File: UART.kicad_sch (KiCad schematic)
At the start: 22 parts, among them J19 430450212, J9 430450612, T1 DA2304-ALD, U5 MAX485, U6 LP2985A-50DBVR, U9 ISO3086TDW

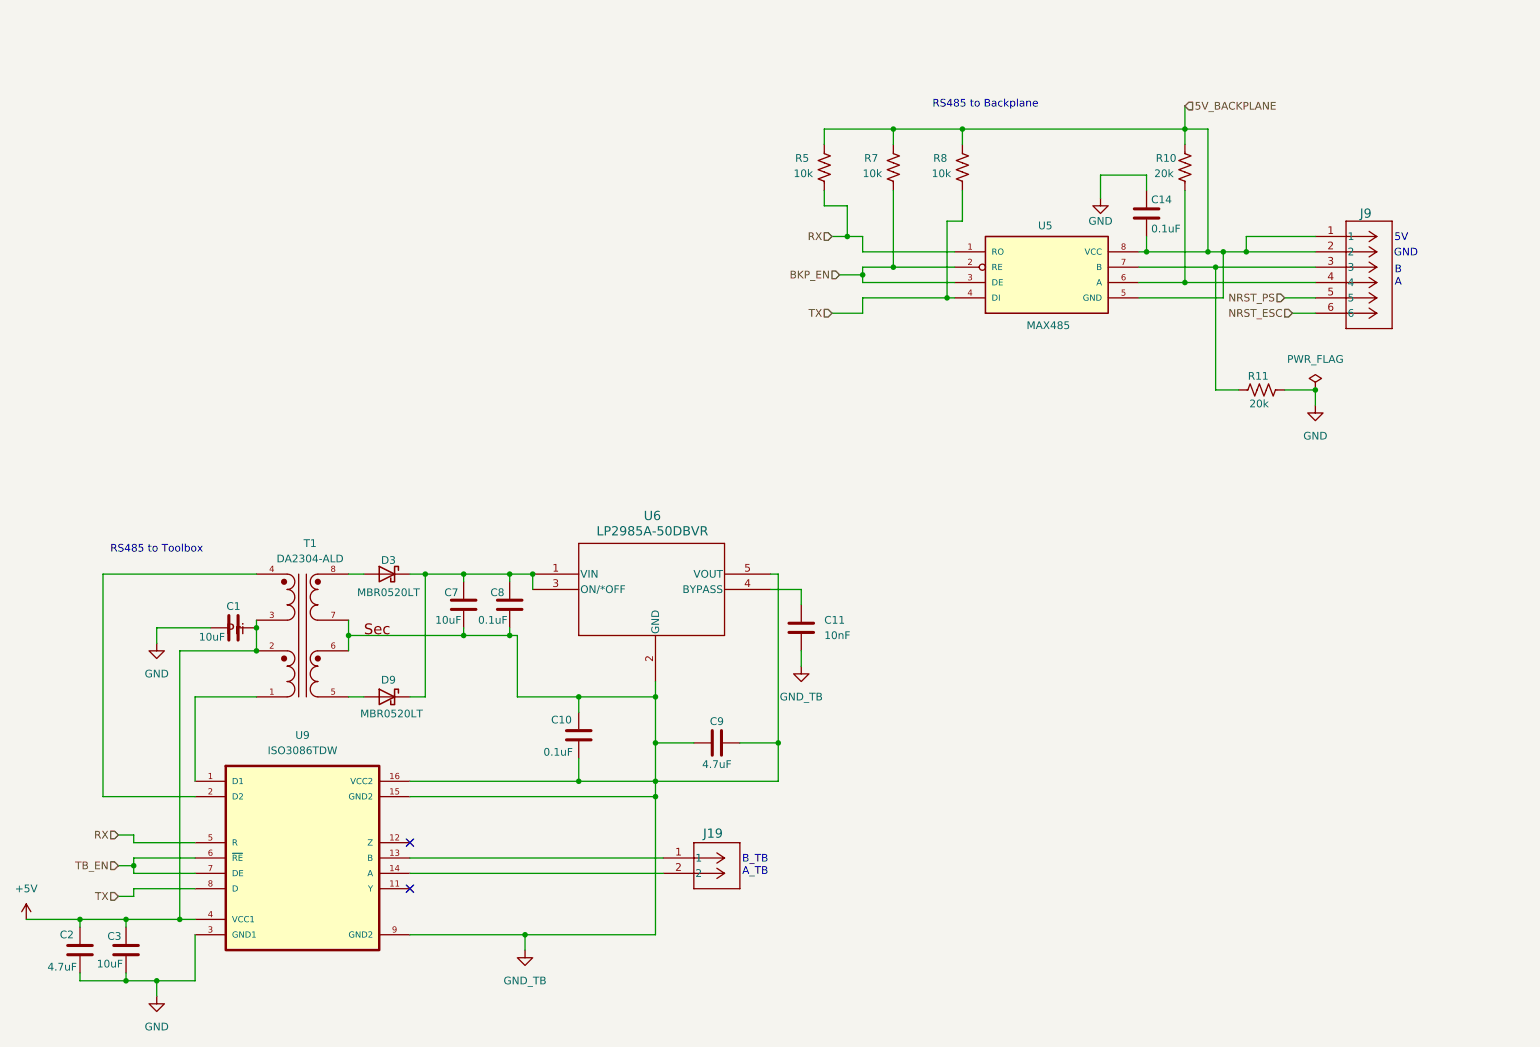
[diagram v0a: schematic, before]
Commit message: Final Schematic Update
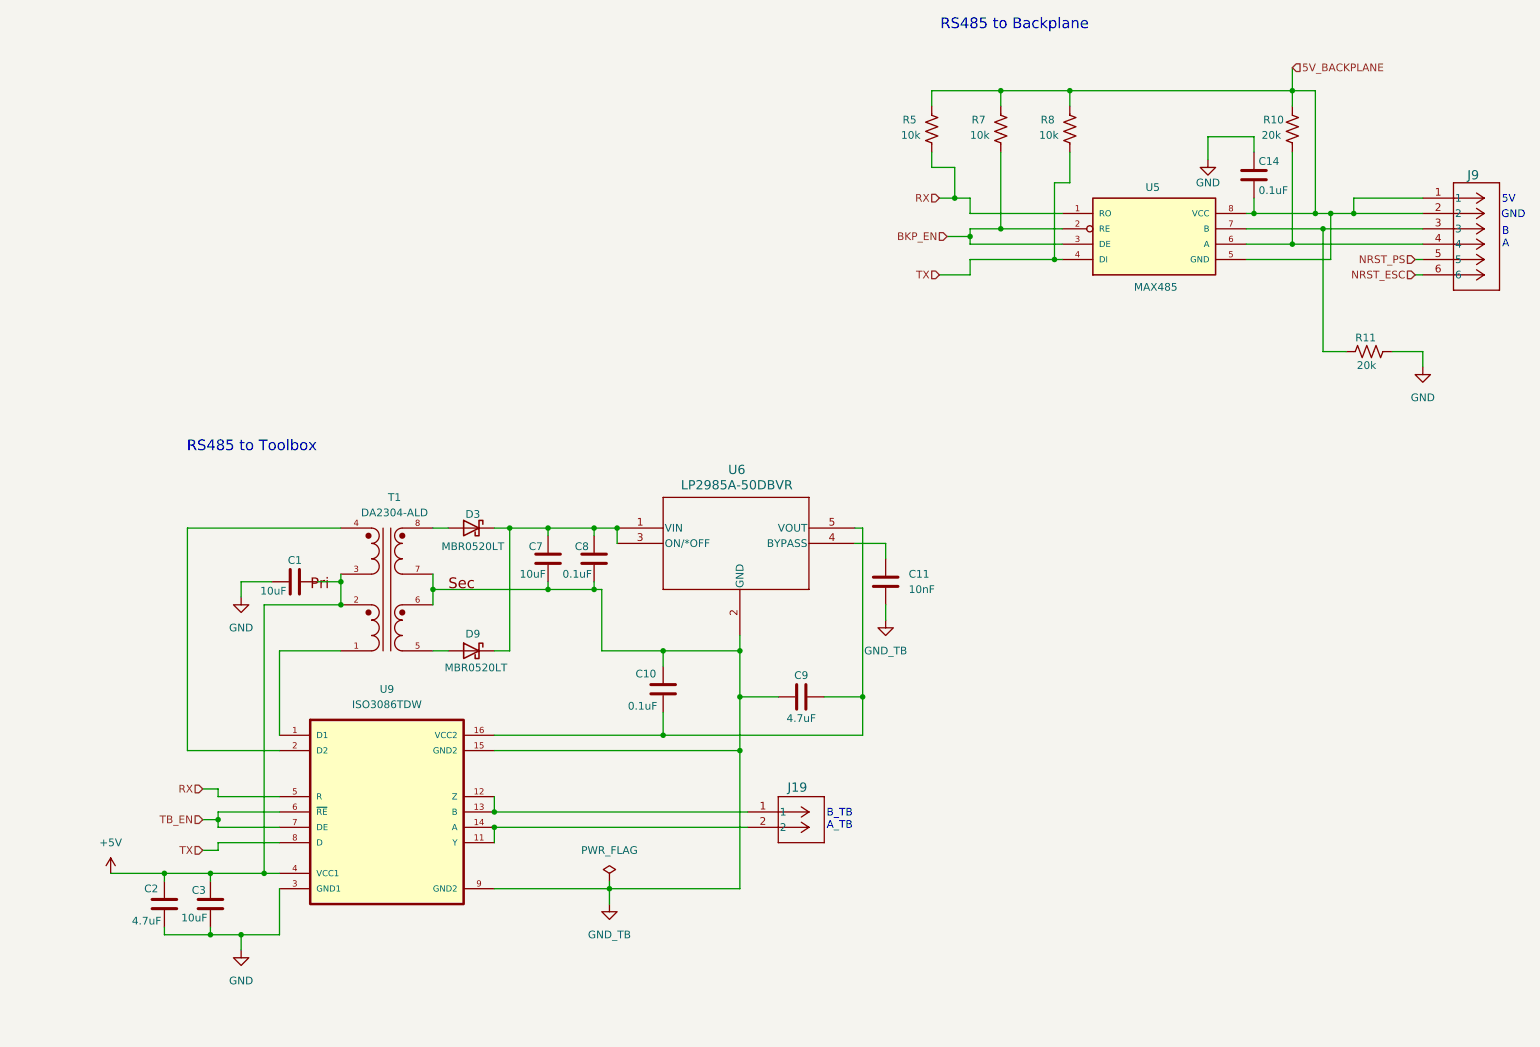
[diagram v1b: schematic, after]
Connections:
- net GND_TB: no longer C10.2, C9.2, U6.5 (VOUT), U9.16 (VCC2)
- net at U9.11 (Y): now also J19.2, U9.14 (A)
- net at U9.12 (Z): now also J19.1, U9.13 (B)
- new net: C10.2, C9.2, U6.5 (VOUT), U9.16 (VCC2)
- no-connect marks 2 -> 0
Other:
- moved on the sheet: C1, C10, C11, C14, C2, C3, C7, C8, C9, D3, D9, J19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
